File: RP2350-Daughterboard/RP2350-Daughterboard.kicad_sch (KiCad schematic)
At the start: 34 parts, among them J1 ISA16_DAUGHTER_BUS, J2 SWD, J5 HDMI_A, SW1 BOOTSEL, SW2 RESET, U1 RP2354B, U2 APS6404L-3SQR-SN, U3 TPD8F003, Y1 12MHz ABM8-272-T3

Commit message: Added Readme introduction
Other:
- moved on the sheet: C1, C10, C2, C3, C4, C5, C6, C7, C8, C9, J1, J2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

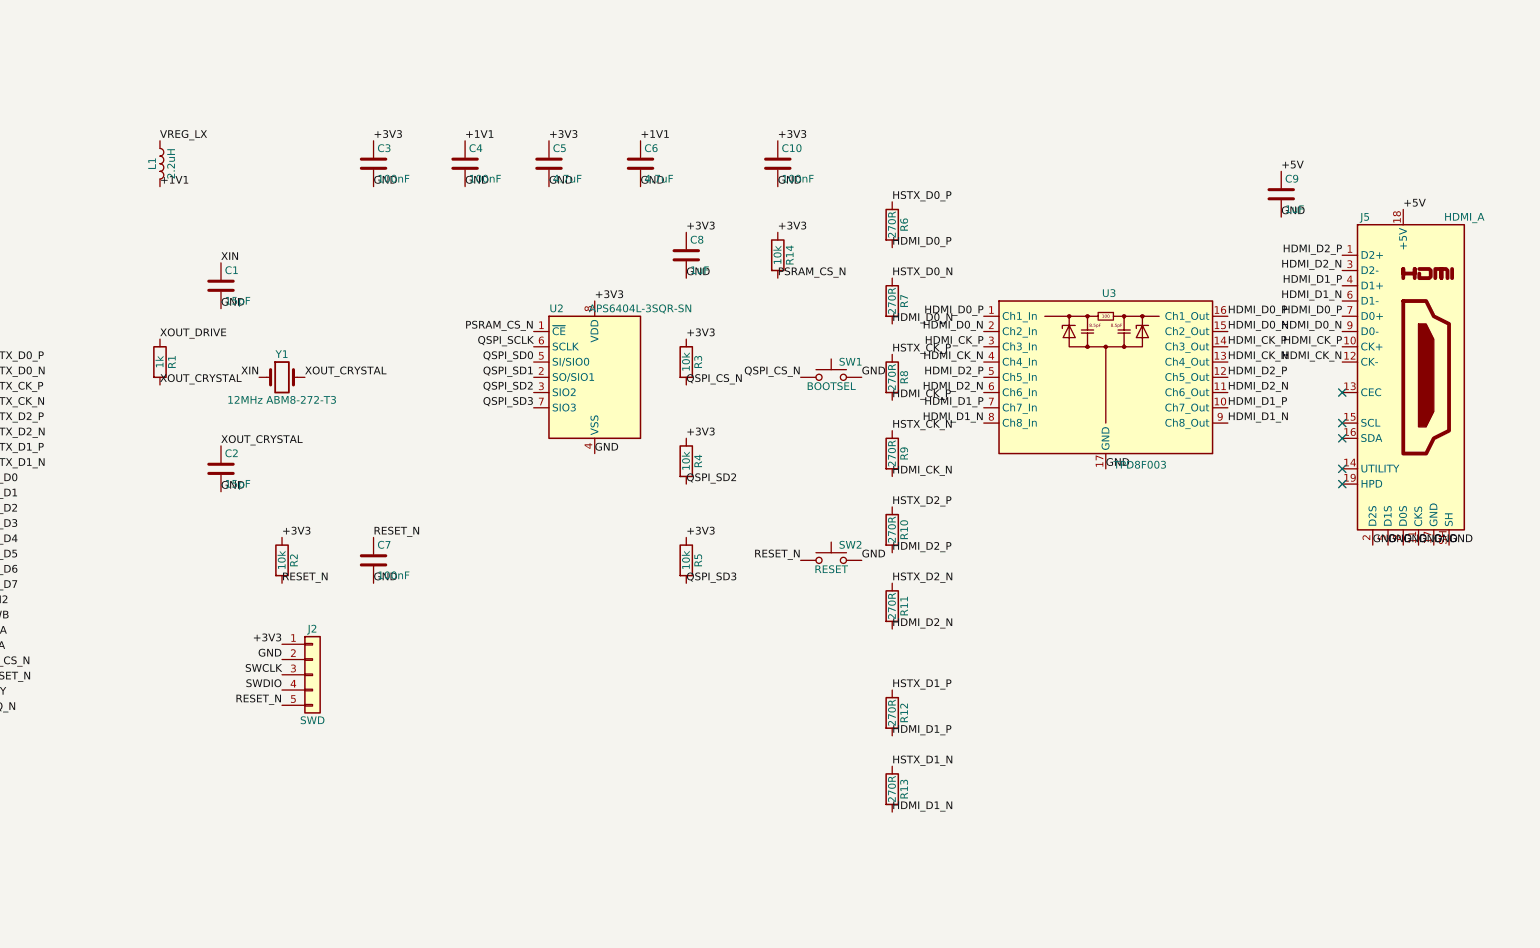
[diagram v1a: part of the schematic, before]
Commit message: Fixed HDMI
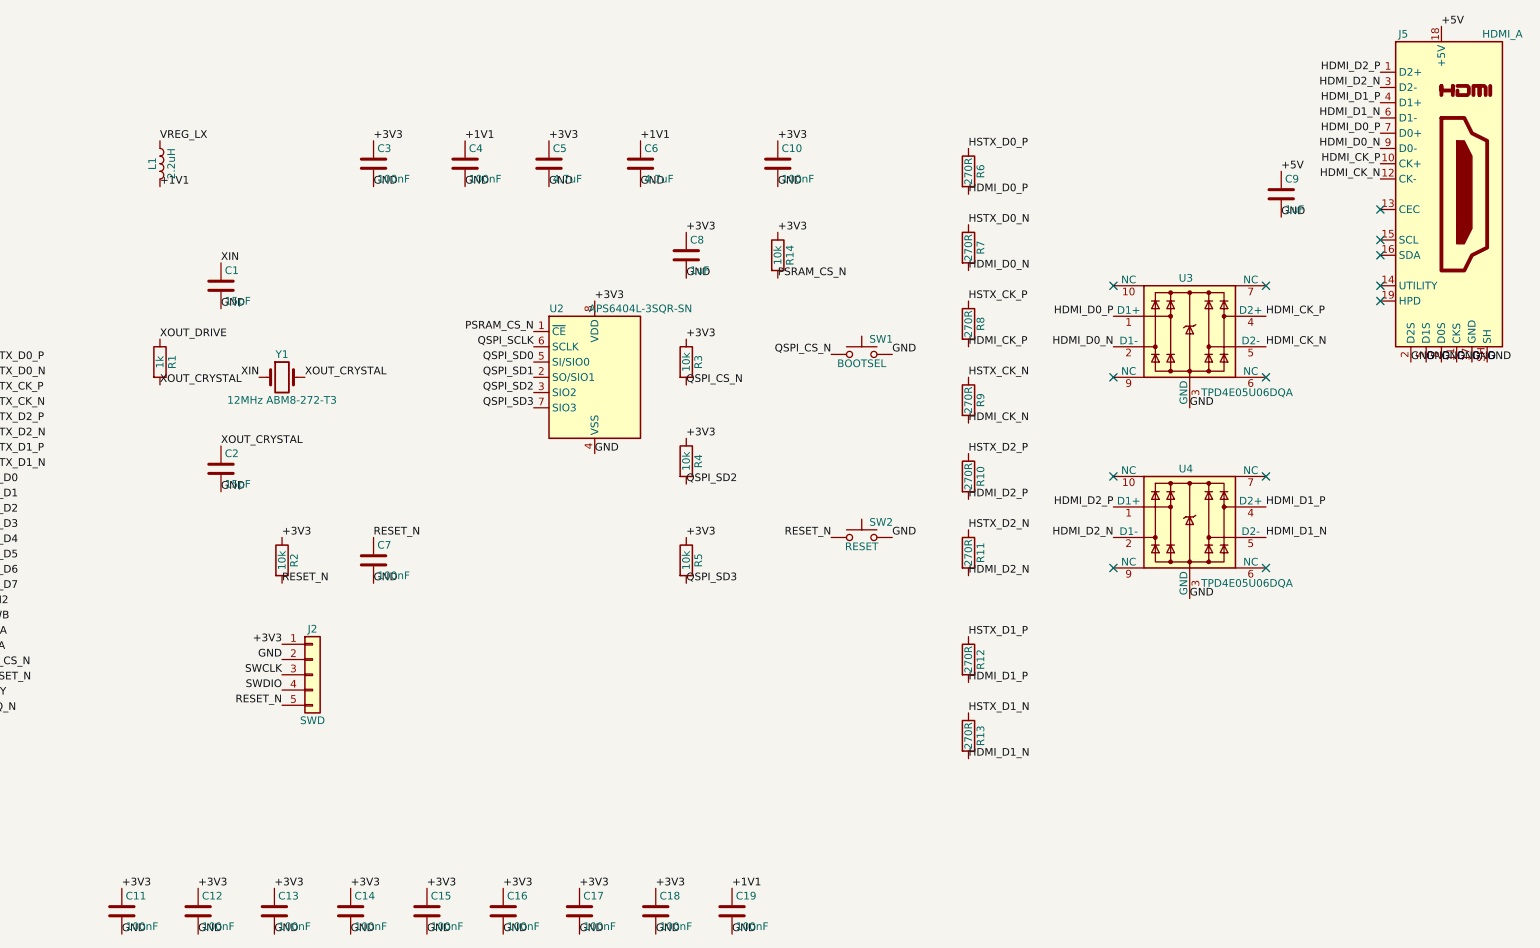
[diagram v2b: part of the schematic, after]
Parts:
- removed U3: TPD8F003, symbol Power_Protection:TPD8F003
- added C11, C12, C13, C14, C15, C16, C17, C18, C19: 100nF, symbol Device:C
- added U3, U4: TPD4E05U06DQA, symbol Power_Protection:TPD4E05U06DQA
- C3, C4, C5, C6: footprint (none) -> Capacitor_SMD:C_0603_1608Metric
- R10, R11, R12, R13, R6, R7, R8, R9: footprint (none) -> Resistor_SMD:R_0603_1608Metric
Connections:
- net +1V1: now also C19.1
- net +3V3: now also C11.1, C12.1, C13.1, C14.1, C15.1, C16.1, C17.1, C18.1
- net GND: now also C11.2, C12.2, C13.2, C14.2, C15.2, C16.2, C17.2, C18.2, C19.2, U3.3 (GND), U3.8 (GND), U4.3 (GND), U4.8 (GND)
- net HDMI_CK_N: now also U3.5 (D2-)
- net HDMI_CK_P: now also U3.4 (D2+)
- net HDMI_D0_N: now also U3.2 (D1-)
- net HDMI_D0_P: now also U3.1 (D1+)
- net HDMI_D1_N: now also U4.5 (D2-)
- net HDMI_D1_P: now also U4.4 (D2+)
- net HDMI_D2_N: now also U4.2 (D1-)
- net HDMI_D2_P: now also U4.1 (D1+)
- no-connect marks 23 -> 31
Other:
- moved on the sheet: J5, R10, R11, R12, R13, R6, R7, R8, R9, SW1, SW2
